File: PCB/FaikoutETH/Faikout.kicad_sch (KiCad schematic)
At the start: 72 parts, among them J1 1x5, J2 TC2030-USB-NL, J3 Reset, J4 RJ45_LED, Q1 BSS138PS, U1 KSZ8851SNL, U4 ESP32-S3-MINI-1, U5 TPS62933, Y1 Crystal_GND24

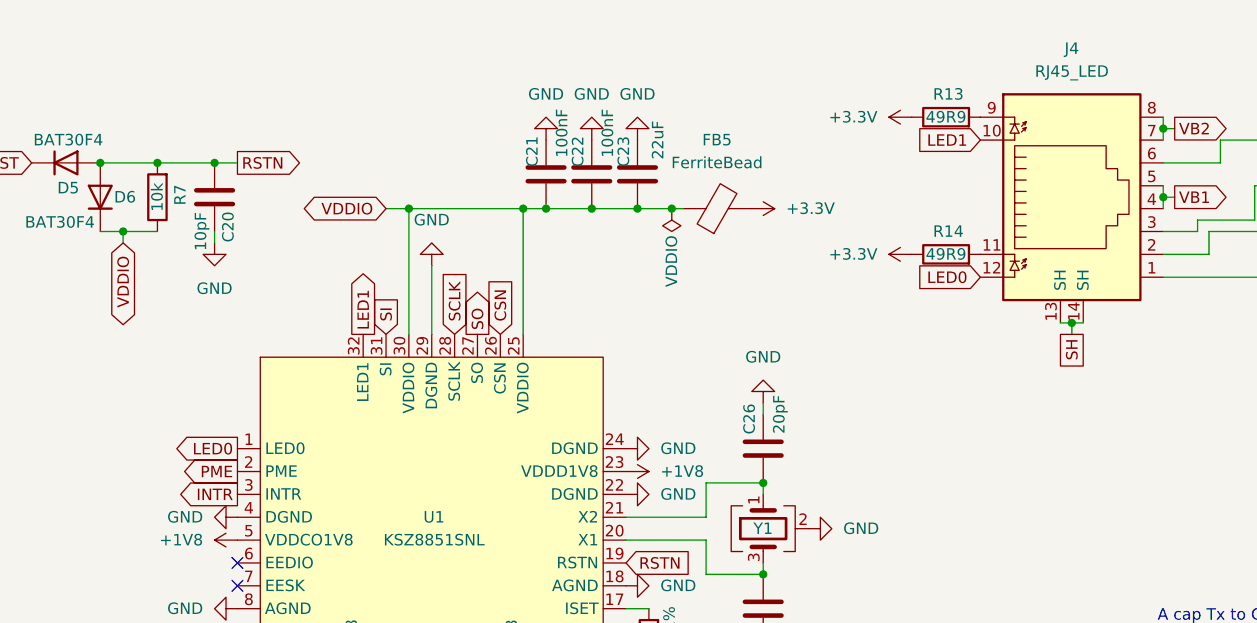
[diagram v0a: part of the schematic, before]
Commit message: New ETH
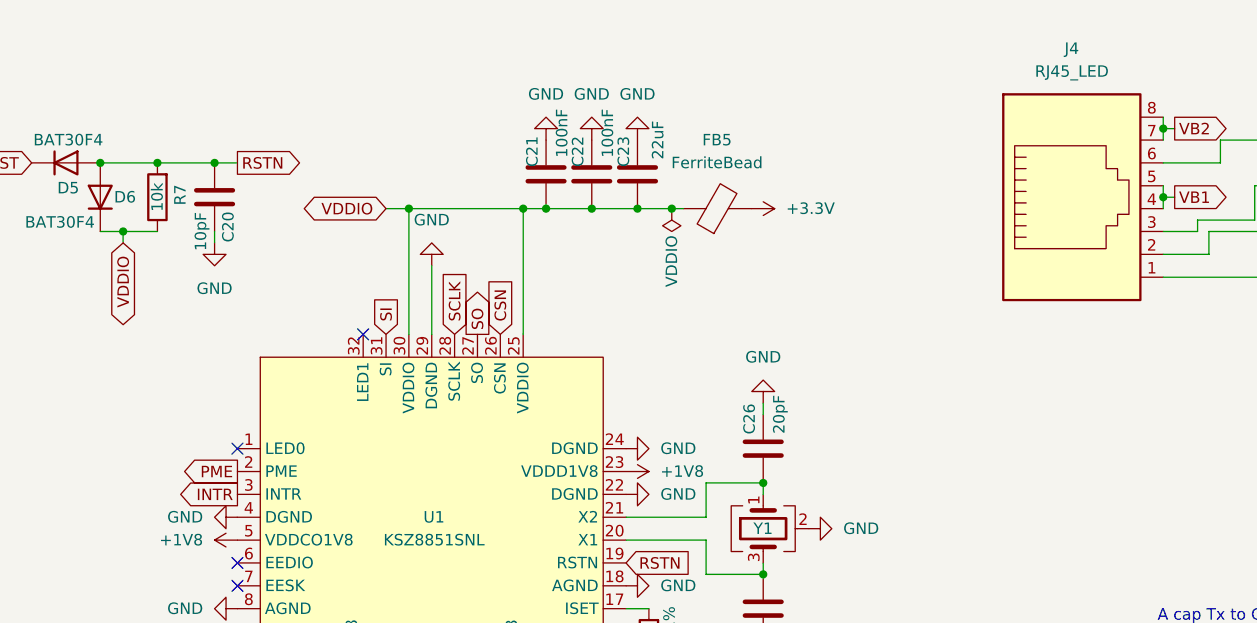
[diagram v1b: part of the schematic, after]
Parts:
- removed R13, R14: 49R9, RevK:R_0201, symbol Device:R
- J4: footprint RevK:HC-WK88-H21-DKH -> RevK:RC01516; symbol RevK:HC-WK88-H21-DKH -> RevK:RC01516; MPN C48618190 -> C708636; Position Offset (none) -> 0,0.5
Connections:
- net LED0: no longer names the net of U1.1 (LED0)
- net LED0: no longer J4.12
- net LED1: no longer names the net of U1.32 (LED1)
- net LED1: no longer J4.10
- removed net SH: J4.13 (SH), J4.14 (SH)
- no-connect marks 28 -> 30
